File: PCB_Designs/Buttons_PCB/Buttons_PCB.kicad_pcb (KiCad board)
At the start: 2 copper layers, 50 x 158.8 mm, 84 parts, among them P1 CONN_02X05, P2 CONN_01X01, P3 CONN_01X01, P4 CONN_01X01, P5 CONN_01X01, U1 CHERRY-MX, U10 CHERRY-MX, U11 CHERRY-MX, U12 CHERRY-MX, U13 MCP23017, U14 MCP23017, U2 CHERRY-MX, U3 CHERRY-MX, U4 CHERRY-MX, U5 CHERRY-MX, U6 CHERRY-MX, U7 CHERRY-MX, U8 CHERRY-MX, U9 CHERRY-MX

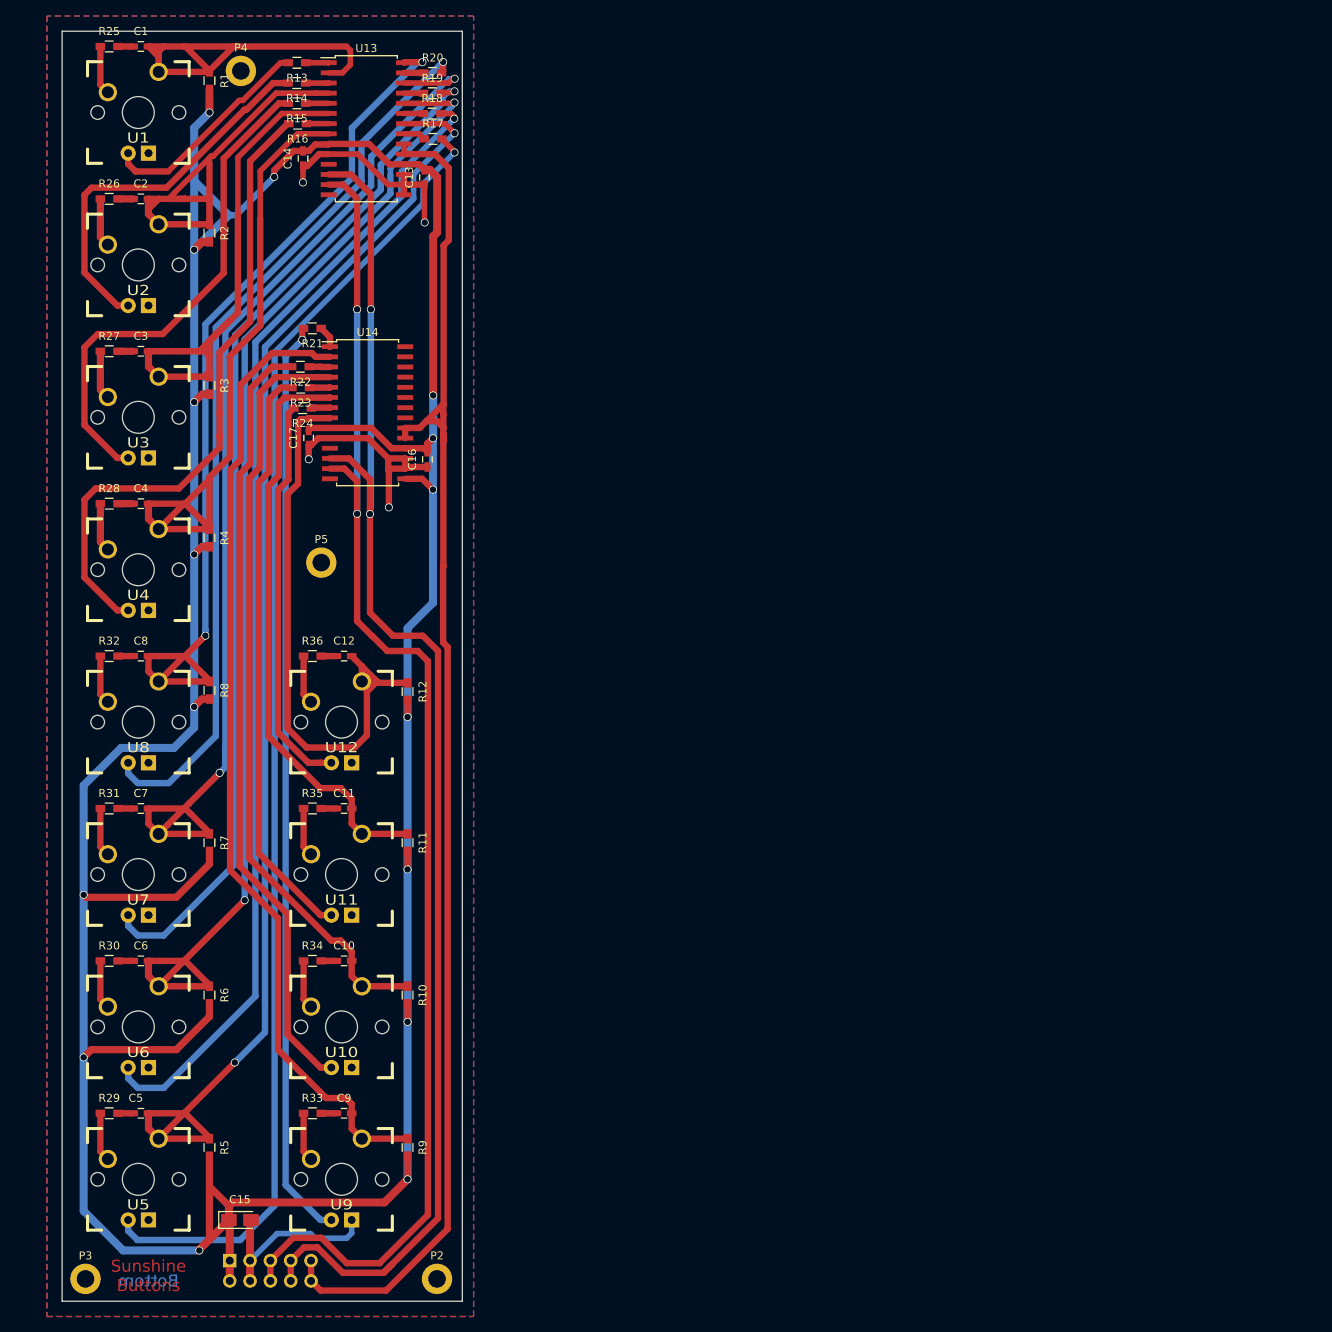
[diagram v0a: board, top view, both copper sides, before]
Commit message: Nya Photomasks Buttons
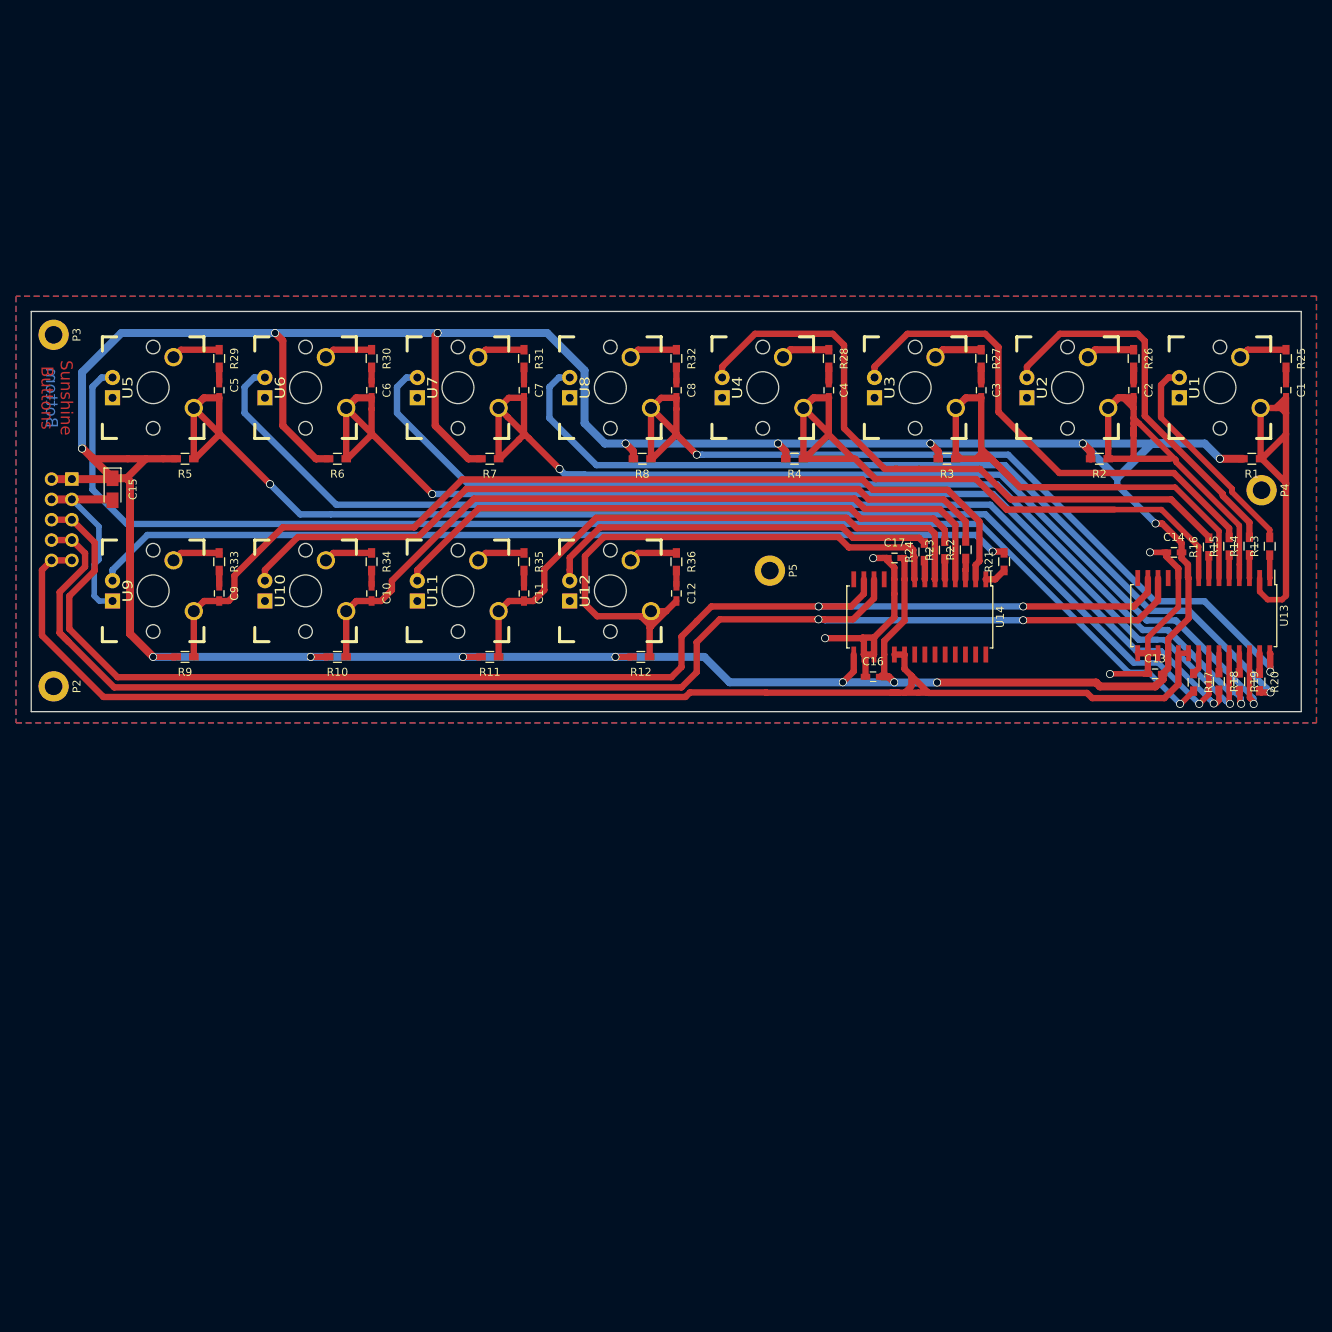
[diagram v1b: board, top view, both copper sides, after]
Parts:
- moved R25 152.2 mm to (217.1, 66.3), turned to 270 degrees
- moved C1 149.5 mm to (217.1, 70.3), turned to 270 degrees
- moved D1 139.5 mm to (208.9, 70.0), turned to 270 degrees
- moved U1 139.5 mm to (208.9, 70.0), turned to 270 degrees
- moved R1 138.6 mm to (212.8, 78.8), turned to 180 degrees
- moved P4 137.9 mm to (214.1, 82.8), turned to 270 degrees
- moved R13 135.8 mm to (215.1, 89.8), turned to 90 degrees
- moved R14 132.4 mm to (212.5, 89.8), turned to 90 degrees
- moved R26 129.6 mm to (198.1, 66.3), turned to 270 degrees
- moved R15 129.0 mm to (210.0, 89.8), turned to 90 degrees
- moved R20 128.4 mm to (213.8, 106.7), turned to 270 degrees
- moved C2 126.4 mm to (198.1, 70.3), turned to 270 degrees
- moved R16 125.6 mm to (207.5, 89.9), turned to 90 degrees
- moved R19 124.8 mm to (211.3, 106.7), turned to 270 degrees
- moved R18 121.3 mm to (208.7, 106.7), turned to 270 degrees
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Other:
- board size 50 x 158.8 mm -> 158.8 x 50 mm
